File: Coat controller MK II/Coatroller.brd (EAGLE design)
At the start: 64.8 x 21.6 mm, 8 parts, among them U1 ATMEGA328P_PDIP, U2 V_REG_LDOSMD, Y1 ABM3B-16.000MHZ-B2-T

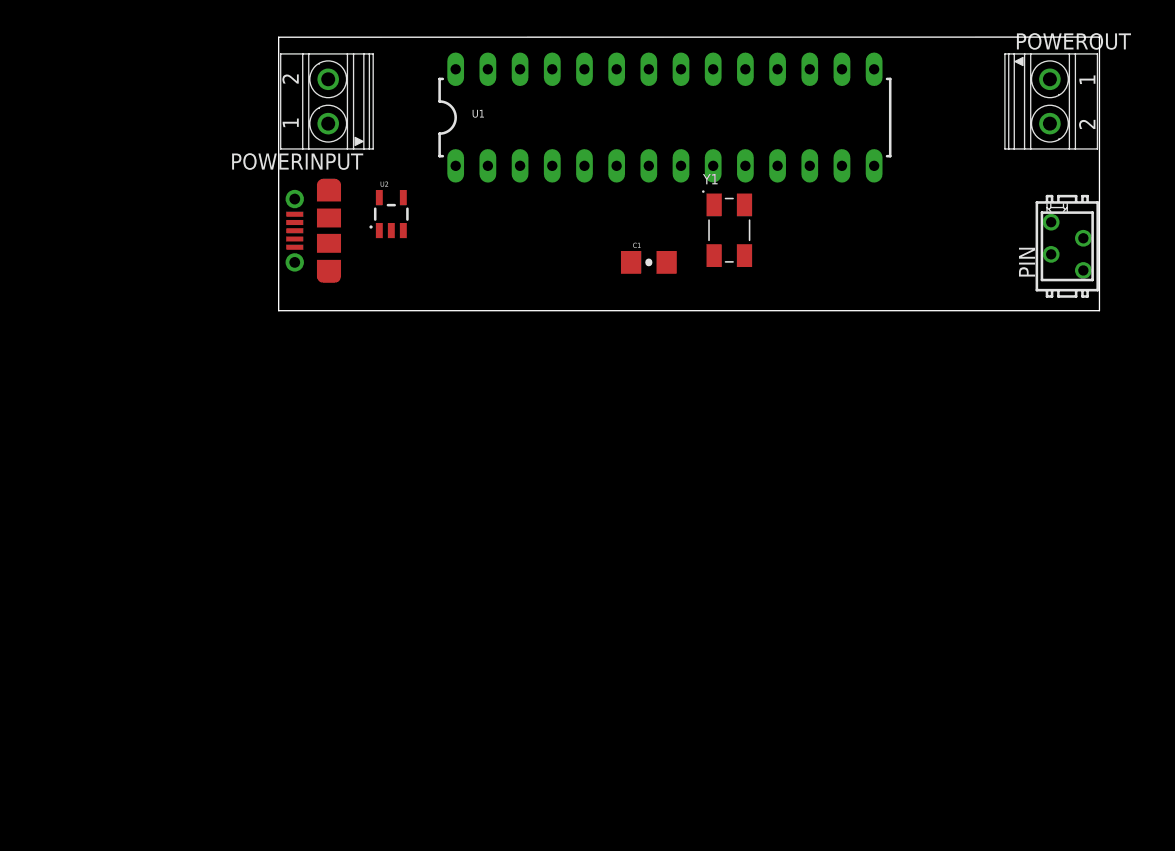
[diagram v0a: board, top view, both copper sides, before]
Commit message: finished placing and routing
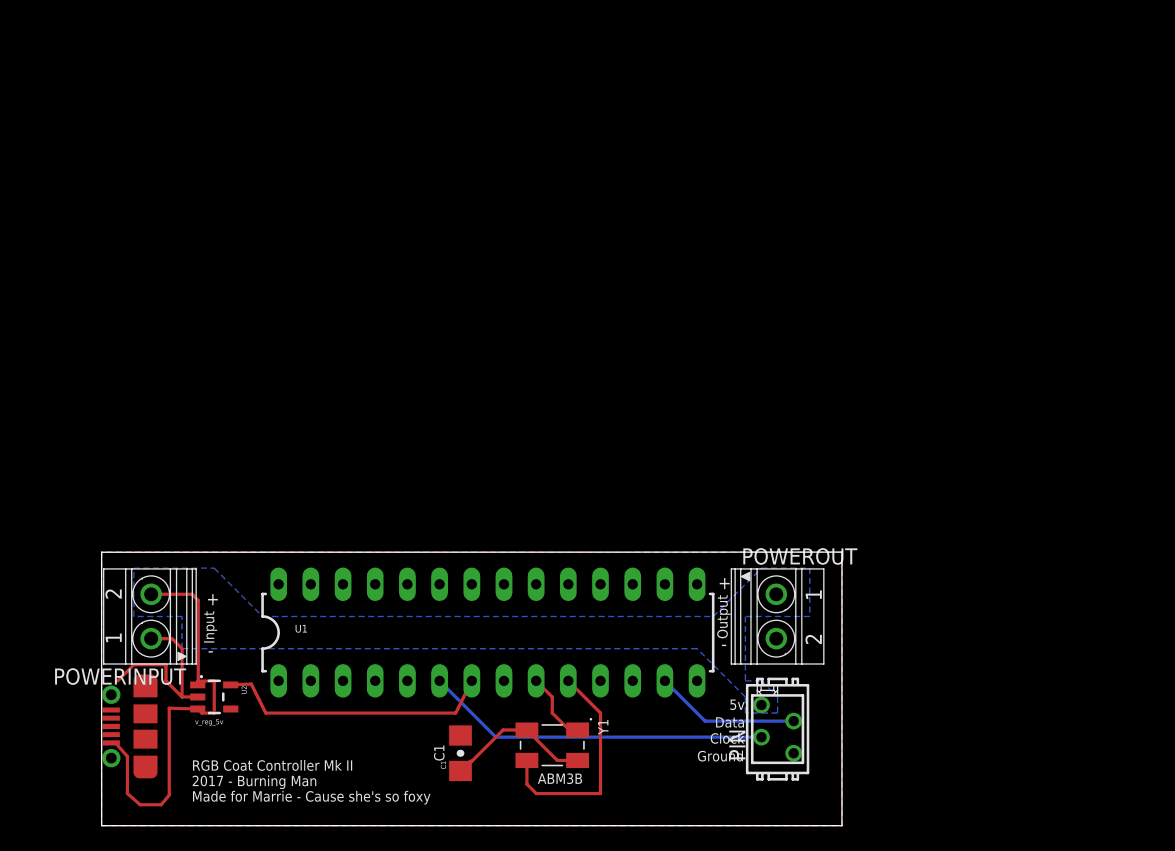
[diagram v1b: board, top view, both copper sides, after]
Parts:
- moved POWEROUT 46.0 mm to (53.3, 16.5)
- moved PIN 44.4 mm to (53.3, 7.62)
- moved POWERINPUT 43.0 mm to (3.81, 16.5)
- moved U1 43.0 mm to (30.5, 15.2)
- moved Y1 43.0 mm to (35.6, 6.35), turned to 270 degrees
- moved U$1 41.7 mm to (0.76, 5.33)
- moved C1 41.5 mm to (28.3, 5.71), turned to 90 degrees
- moved U2 40.6 mm to (8.89, 10.2), turned to 270 degrees
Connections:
- removed net N$4: PIN.3, U1.13
- removed net N$5: PIN.2, U1.4
- new net CLOCK: PIN.3, U1.6
- new net DATA: PIN.2, U1.13
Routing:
- net VCC: track 0.00 -> 34.0 mm
- net CLOCK: track 0.00 -> 27.2 mm
- net 5V: track 0.00 -> 22.0 mm
- net N$2: track 0.00 -> 17.9 mm
- net GROUND: track 0.00 -> 15.2 mm
- net N$3: track 0.00 -> 11.6 mm
- net DATA: track 0.00 -> 11.5 mm
- net N$1: track 0.00 -> 5.72 mm
- added copper zone on layer 1, net GROUND
- added copper zone on layer 16, net VCC
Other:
- board size 64.8 x 21.6 mm -> 58.4 x 21.6 mm
- board text added: "+"
- board text added: "-"
- board text added: "5v"
- board text added: "ABM3B"
- board text added: "C1"
- board text added: "Clock"
- board text added: "Data"
- board text added: "Ground"
- board text added: "Input"
- board text added: "Made by Remington Winters"
- board text added: "Output"
- board text added: "RGB Coat Controller Mk II 2017 - Burning Man Made for Marrie - Cause she's so foxy"
- board text added: "v_reg_5v"
